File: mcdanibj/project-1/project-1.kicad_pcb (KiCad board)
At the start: 2 copper layers, 7 parts, among them J1 Conn_01x04

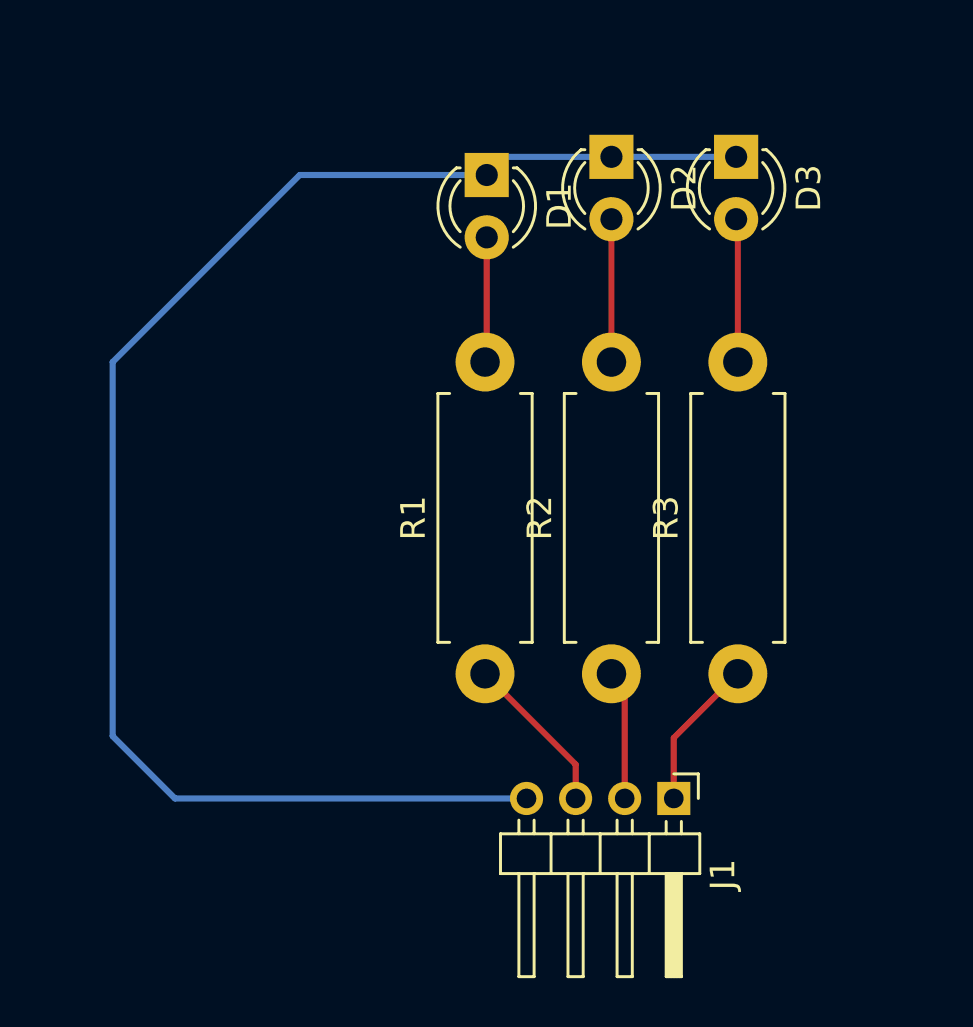
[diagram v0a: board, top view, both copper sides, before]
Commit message: aaaaa
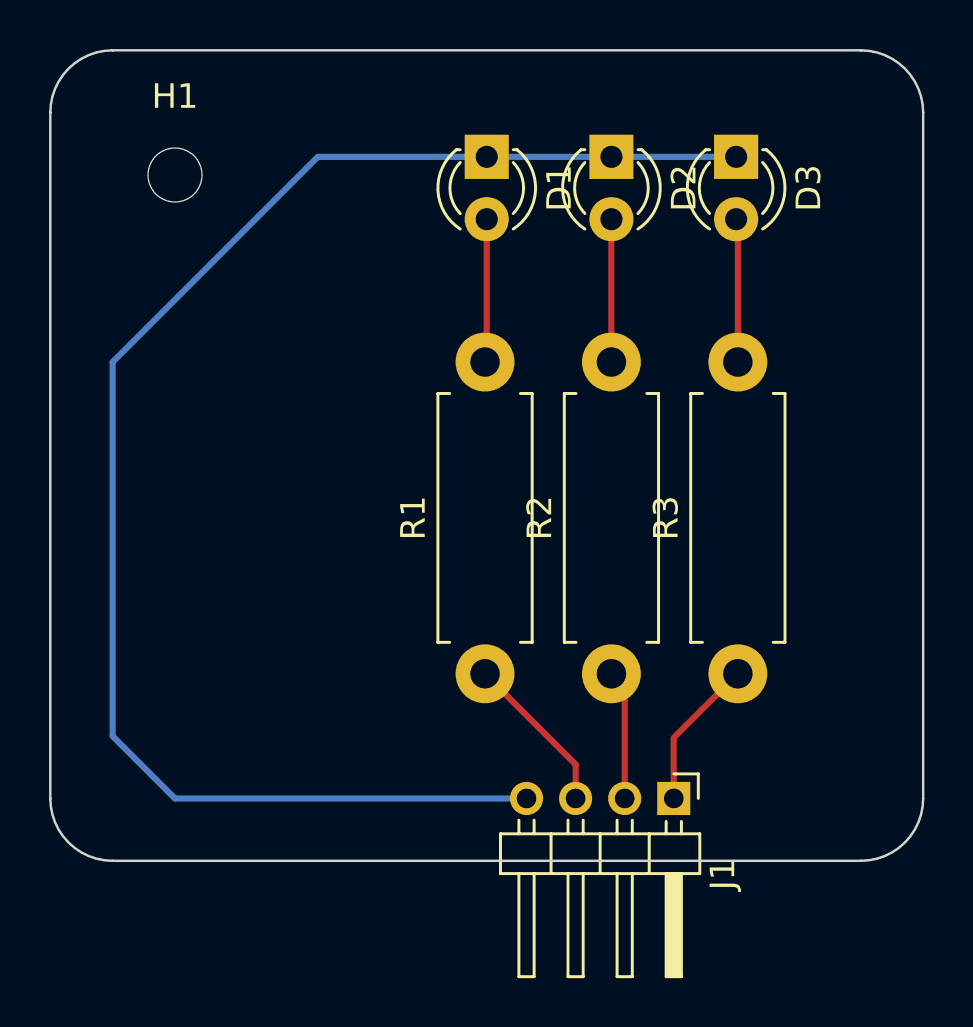
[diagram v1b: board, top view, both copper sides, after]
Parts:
- added H1: MountingHole, MountingHole:MountingHole_2.2mm_M2, F.Cu at (127.0, 73.7)
- moved D1 0.74 mm to (139.7, 72.9)
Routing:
- net Net-(D1-K): track 62.0 -> 63.1 mm
- net Net-(D1-A): track 5.11 -> 5.85 mm
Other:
- board outline added: 35.6 x 33 mm
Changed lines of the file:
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@@
     )
+  )
+  (footprint "MountingHole:MountingHole_2.2mm_M2" (layer "F.Cu")
+    (at 127 73.66)
+    (descr "Mounting Hole 2.2mm, no annular, M2")
+    (tags "mounting hole 2.2mm no annular m2")
+    (property "Sheetfile" "project-1.kicad_sch")
+    (property "Sheetname" "")
+    (property "ki_description" "Mounting Hole without connection")
+    (property "ki_keywords" "mounting hole")
+    (attr exclude_from_pos_files)
+    (fp_text reference "H1" (at 0 -3.2) (layer "F.SilkS")
+        (effects (font (size 1 1) (thickness 0.15)))
+    )
+    (fp_text value "MountingHole" (at 0 3.2) (layer "F.Fab")
+        (effects (font (size 1 1) (thickness 0.15)))
+    )
+    (fp_text user "${REFERENCE}" (at 0 0) (layer "F.Fab")
+        (effects (font (size 1 1) (thickness 0.15)))
+    )
+    (fp_circle (center 0 0) (end 2.2 0)
+      (stroke (width 0.15) (type solid)) (fill none) (layer "Cmts.User"))
+    (fp_circle (center 0 0) (end 2.45 0)
+      (stroke (width 0.05) (type solid)) (fill none) (layer "F.CrtYd"))
+    (pad "" np_thru_hole circle (at 0 0) (size 2.2 2.2) (drill 2.2) (layers "*.Cu" "*.Mask"))
   )
   (footprint "Resistor_THT:R_Axial_DIN0411_L9.9mm_D3.6mm_P12.70mm_Horizontal" (layer "F.Cu")
@@
   )
   (footprint "LED_THT:LED_D3.0mm" (layer "F.Cu")
-    (at 139.7 73.66 -90)
+    (at 139.7 72.92 -90)
     (descr "LED, diameter 3.0mm, 2 pins")
     (tags "LED diameter 3.0mm 2 pins")
@@
     )
   )
+  (gr_arc (start 154.94 68.58) (mid 156.736051 69.323949) (end 157.48 71.12)
+    (stroke (width 0.1) (type default)) (layer "Edge.Cuts"))
+  (gr_line (start 157.48 99.06) (end 157.48 71.12)
+    (stroke (width 0.1) (type default)) (layer "Edge.Cuts"))
+  (gr_line (start 124.46 101.6) (end 154.94 101.6)
+    (stroke (width 0.1) (type default)) (layer "Edge.Cuts"))
+  (gr_line (start 154.94 68.58) (end 124.46 68.58)
+    (stroke (width 0.1) (type default)) (layer "Edge.Cuts"))
+  (gr_arc (start 157.48 99.06) (mid 156.736051 100.856051) (end 154.94 101.6)
+    (stroke (width 0.1) (type default)) (layer "Edge.Cuts"))
+  (gr_arc (start 124.46 101.6) (mid 122.663949 100.856051) (end 121.92 99.06)
+    (stroke (width 0.1) (type default)) (layer "Edge.Cuts"))
+  (gr_arc (start 121.92 71.12) (mid 122.663949 69.323949) (end 124.46 68.58)
+    (stroke (width 0.1) (type default)) (layer "Edge.Cuts"))
+  (gr_line (start 121.92 99.06) (end 121.92 71.12)
+    (stroke (width 0.1) (type default)) (layer "Edge.Cuts"))
+  (segment (start 127 99.06) (end 141.32 99.06) (width 0.25) (layer "B.Cu") (net 1))
+  (segment (start 139.7 72.92) (end 132.82 72.92) (width 0.25) (layer "B.Cu") (net 1))
   (segment (start 124.46 81.28) (end 124.46 96.52) (width 0.25) (layer "B.Cu") (net 1))
-  (segment (start 124.46 96.52) (end 127 99.06) (width 0.25) (layer "B.Cu") (net 1))
-  (segment (start 132.08 73.66) (end 124.46 81.28) (width 0.25) (layer "B.Cu") (net 1))
-  (segment (start 144.78 72.92) (end 140.44 72.92) (width 0.25) (layer "B.Cu") (net 1))
+  (segment (start 124.46 81.28) (end 132.82 72.92) (width 0.25) (layer "B.Cu") (net 1))
   (segment (start 149.86 72.92) (end 144.78 72.92) (width 0.25) (layer "B.Cu") (net 1))
   (segment (start 140.44 72.92) (end 139.7 73.66) (width 0.25) (layer "B.Cu") (net 1))
-  (segment (start 127 99.06) (end 141.32 99.06) (width 0.25) (layer "B.Cu") (net 1))
-  (segment (start 139.7 73.66) (end 132.08 73.66) (width 0.25) (layer "B.Cu") (net 1))
-  (segment (start 139.7 76.2) (end 139.7 81.21) (width 0.25) (layer "F.Cu") (net 2))
+  (segment (start 124.46 96.52) (end 127 99.06) (width 0.25) (layer "B.Cu") (net 1))
+  (segment (start 144.78 72.92) (end 139.7 72.92) (width 0.25) (layer "B.Cu") (net 1))
+  (segment (start 139.7 75.46) (end 139.7 81.21) (width 0.25) (layer "F.Cu") (net 2))
   (segment (start 139.7 81.21) (end 139.63 81.28) (width 0.25) (layer "F.Cu") (net 2))
   (segment (start 144.78 81.28) (end 144.78 75.46) (width 0.25) (layer "F.Cu") (net 3))
